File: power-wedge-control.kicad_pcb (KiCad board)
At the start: 2 copper layers, 53.3 x 68.6 mm, 63 parts, among them J1 Conn_01x02, J2 Conn_01x03, J3 Conn_01x02, J4 Conn_01x03, J5 Conn_01x03, J6 Conn_01x06_Female, J7 Conn_01x04_Female, Q1 MMBT3904L, Q2 DMP3099L, Q3 MMBT3904L, Q4 DMP3099L, Q5 MMBT3904L, Q6 MMBT3904L, U1 LM7805_TO220, U2 NC7WZ14P6X

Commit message: Fix hardware debounce circuit (was incorrect).
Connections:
- U2 pad 1: /HWDebounce/SW1IN -> Net-(C10-Pad1)
- U2 pad 3: /HWDebounce/SW2IN -> Net-(C11-Pad1)
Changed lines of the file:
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@@
     (fp_line (start 0.675 -1.1) (end -0.175 -1.1) (layer "F.Fab") (width 0.1))
     (pad "1" smd rect locked (at -0.95 -0.65 270) (size 0.65 0.4) (layers "F.Cu" "F.Paste" "F.Mask")
-      (net 85 "/HWDebounce/SW1IN") (pinfunction "A1") (pintype "input"))
+      (net 70 "Net-(C10-Pad1)") (pinfunction "A1") (pintype "input"))
     (pad "2" smd rect locked (at -0.95 0 270) (size 0.65 0.4) (layers "F.Cu" "F.Paste" "F.Mask")
       (net 1 "GND") (pinfunction "GND") (pintype "passive"))
     (pad "3" smd rect locked (at -0.95 0.65 270) (size 0.65 0.4) (layers "F.Cu" "F.Paste" "F.Mask")
-      (net 86 "/HWDebounce/SW2IN") (pinfunction "A2") (pintype "input"))
+      (net 84 "Net-(C11-Pad1)") (pinfunction "A2") (pintype "input"))
     (pad "4" smd rect locked (at 0.95 0.65 270) (size 0.65 0.4) (layers "F.Cu" "F.Paste" "F.Mask")
       (net 90 "Net-(R20-Pad2)") (pinfunction "Y2") (pintype "output"))

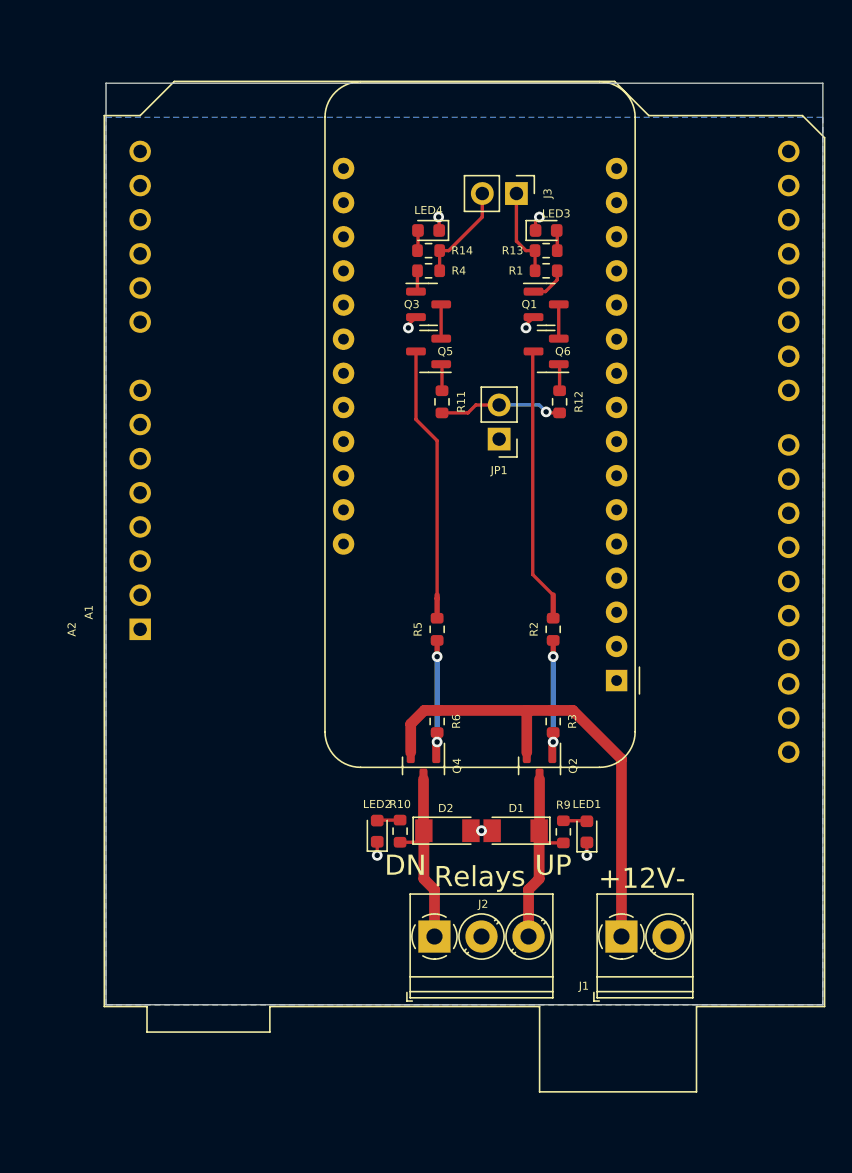
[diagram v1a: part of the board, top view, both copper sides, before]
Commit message: Flip Arduino UNO R3 footprint.
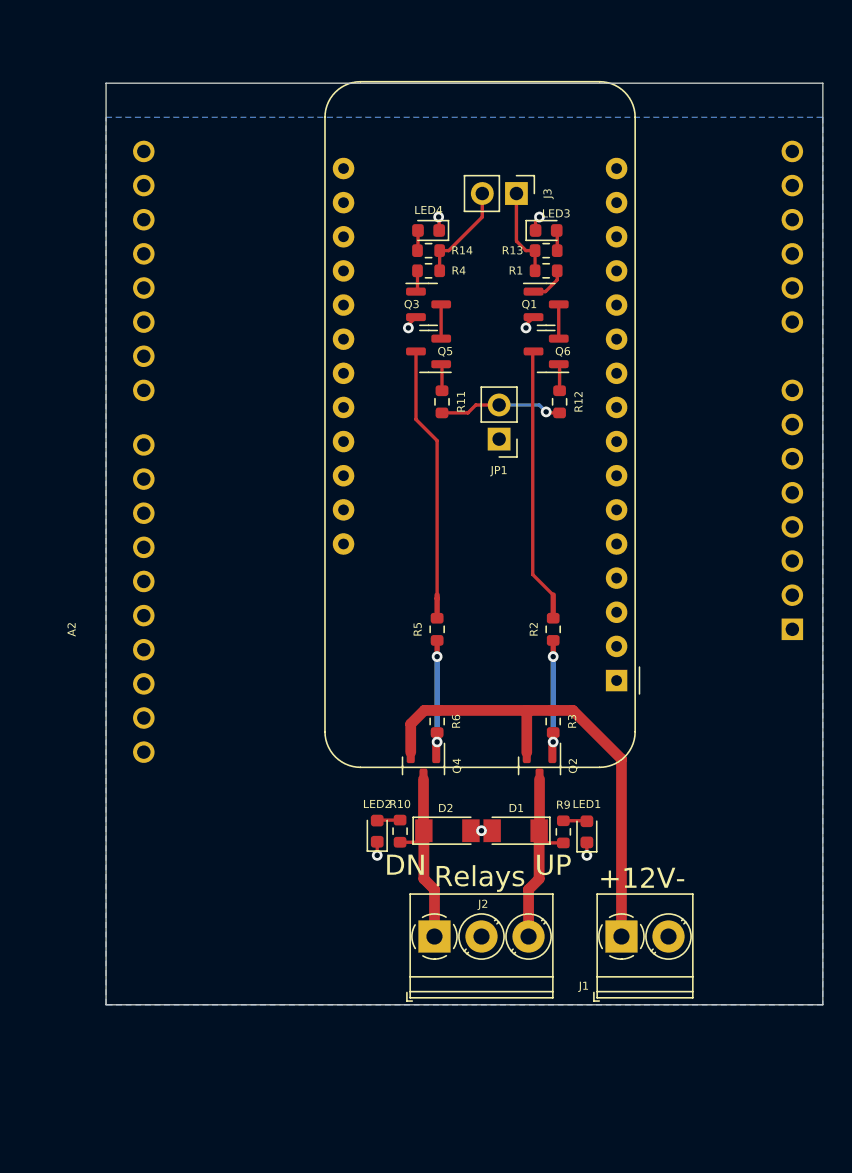
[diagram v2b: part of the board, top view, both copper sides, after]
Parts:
- A1: moved to B.Cu
- moved A1 48.5 mm to (179.1, 91.4)
